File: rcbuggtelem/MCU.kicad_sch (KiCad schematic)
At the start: 29 parts, among them J3 Micro_SD_Card, J4 USB_B_Micro, J5 Conn_01x04_Pin, SW1 SW_Push, U1 ESP32-S3-MINI-1

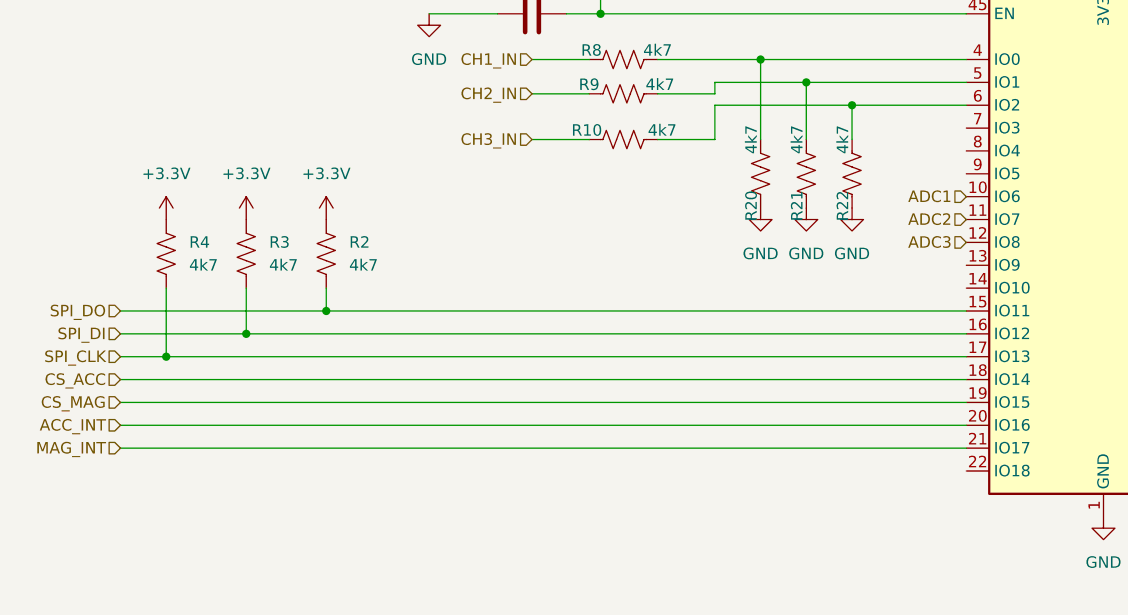
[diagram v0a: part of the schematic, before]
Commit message: up
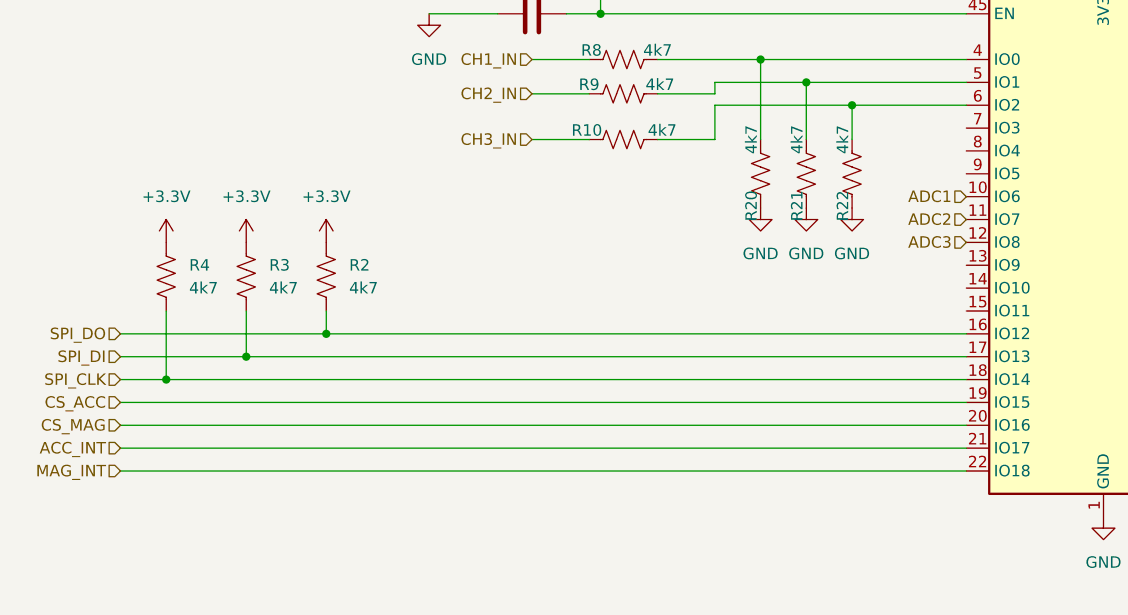
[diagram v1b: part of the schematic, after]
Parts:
- D5: footprint LED_SMD:LED_0603_1608Metric_Pad1.05x0.95mm_HandSolder -> LED_SMD:LED_1206_3216Metric_Pad1.42x1.75mm_HandSolder
- D6: footprint LED_SMD:LED_1206_3216Metric -> LED_SMD:LED_1206_3216Metric_Pad1.42x1.75mm_HandSolder
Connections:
- net ACC_INT: now also U1.21 (IO17); no longer U1.20 (IO16)
- net CS_ACC: now also U1.19 (IO15); no longer U1.18 (IO14)
- net CS_MAG: now also U1.20 (IO16); no longer U1.19 (IO15)
- net MAG_INT: now also U1.22 (IO18); no longer U1.21 (IO17)
- net SPI_CLK: now also U1.18 (IO14); no longer U1.17 (IO13)
- net SPI_DI: now also U1.17 (IO13); no longer U1.16 (IO12)
- net SPI_DO: now also U1.16 (IO12); no longer U1.15 (IO11)
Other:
- moved on the sheet: R2, R3, R4
